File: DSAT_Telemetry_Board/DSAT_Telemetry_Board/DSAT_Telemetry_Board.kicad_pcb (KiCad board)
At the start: 4 copper layers, 73.2 x 96.7 mm, 79 parts, among them IC1 CG2409X3-C2, J1 Conn_01x04_Female, J2 Conn_Coaxial, J3 Conn_01x02_Female, J5 Conn_01x04_Male, SW1 SW_Push, SW2 SW_SPDT, U1 AZ1084-3.3, U5 STM32L433RCTx, U6 Si4463, U7 PSA4-5043+, U8 Watchdog_Timer, Y1 16MHz, Y2 30MHz

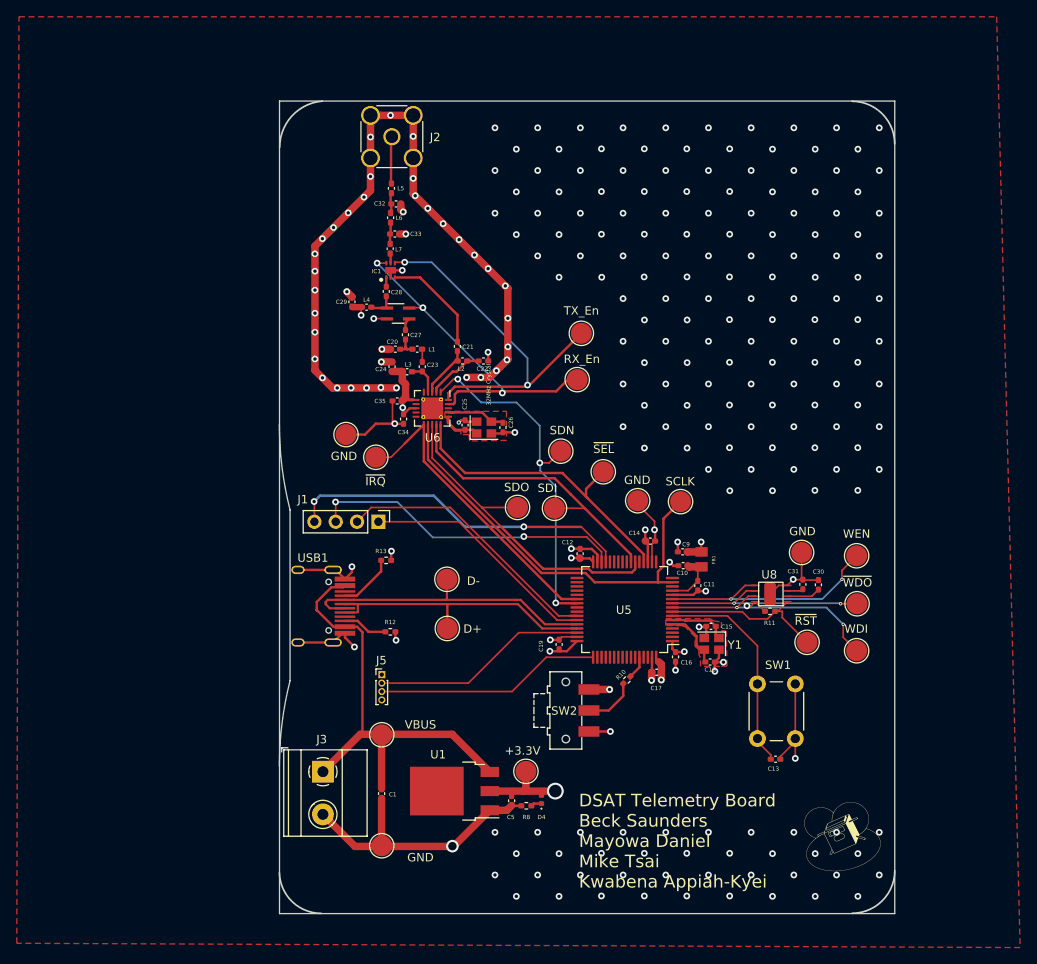
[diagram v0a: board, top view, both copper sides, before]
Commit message: done
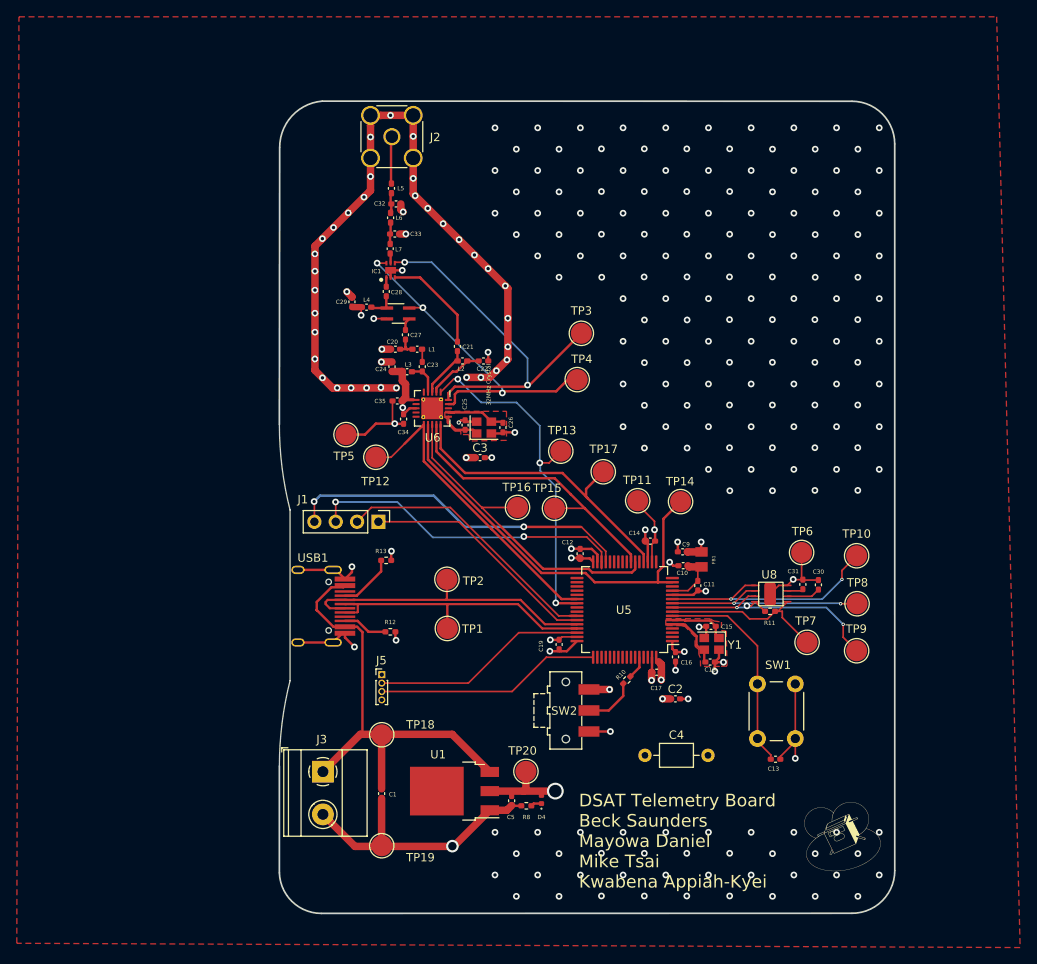
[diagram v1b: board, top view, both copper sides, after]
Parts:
- added C2: 1uF, Capacitor_SMD:C_0402_1005Metric_Pad0.74x0.62mm_HandSolder, F.Cu at (194.2, 123.8)
- added C3: 1uF, Capacitor_SMD:C_0402_1005Metric_Pad0.74x0.62mm_HandSolder, F.Cu at (170.9, 95.1)
- added C4: 100uF, Capacitor_THT:C_Axial_L3.8mm_D2.6mm_P7.50mm_Horizontal, F.Cu at (190.6, 130.5)
- renumbered D+ to TP1, WEN to TP10, GND to TP11, ~{IRQ} to TP12, SDN to TP13, SCLK to TP14, SDI to TP15, SDO to TP16, ~{SEL} to TP17, VBUS to TP18, GND to TP19, D- to TP2, +3.3V to TP20, TX_En to TP3, RX_En to TP4, GND to TP5, GND to TP6, ~{RST} to TP7, ~{WDO} to TP8, WDI to TP9
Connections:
- C27 pad 1: /Transceiver1/TX_Transceiver -> /Low Noise Amplifier1/TX_Transciever
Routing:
- net +3.3V: track 46.3 -> 48.4 mm, vias 11 -> 13
- net GND: track 218.6 -> 220.3 mm, vias 65 -> 67
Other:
- board size 73.2 x 96.7 mm -> 73.2 x 96.6 mm
